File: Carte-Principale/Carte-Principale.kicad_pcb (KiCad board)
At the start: 2 copper layers, 82 parts, among them J1 Serial, J10 5V, J11 Encodeur_G, J12 Encodeur_D, J13 Moteur_Gauche, J14 Moteur_Droit, J15 PCA9685, J16 AX12, J17 I2C_Sensors, J18 LCD_TFT, J19 LCD_SD, J2 PA, J3 PG, J4 SPI2, J5 SPI3, J6 I2C2, J7 I2C3, J8 12V, J9 12VA, Q1 IRF630, Q2 BSS138, Q3 BSS138, Q4 BSS138, Q5 BSS138, SW1 RESET, SW2 Vert, SW3 Jaune, SW4 Bleu, SW5 Rouge, U1 NUCLEOH723ZG, U2 AM26LV32xD, U3 74LVC1G3157, U4 74LVC1G3157, U5 74LVC1G3157, U6 74LVC1G3157

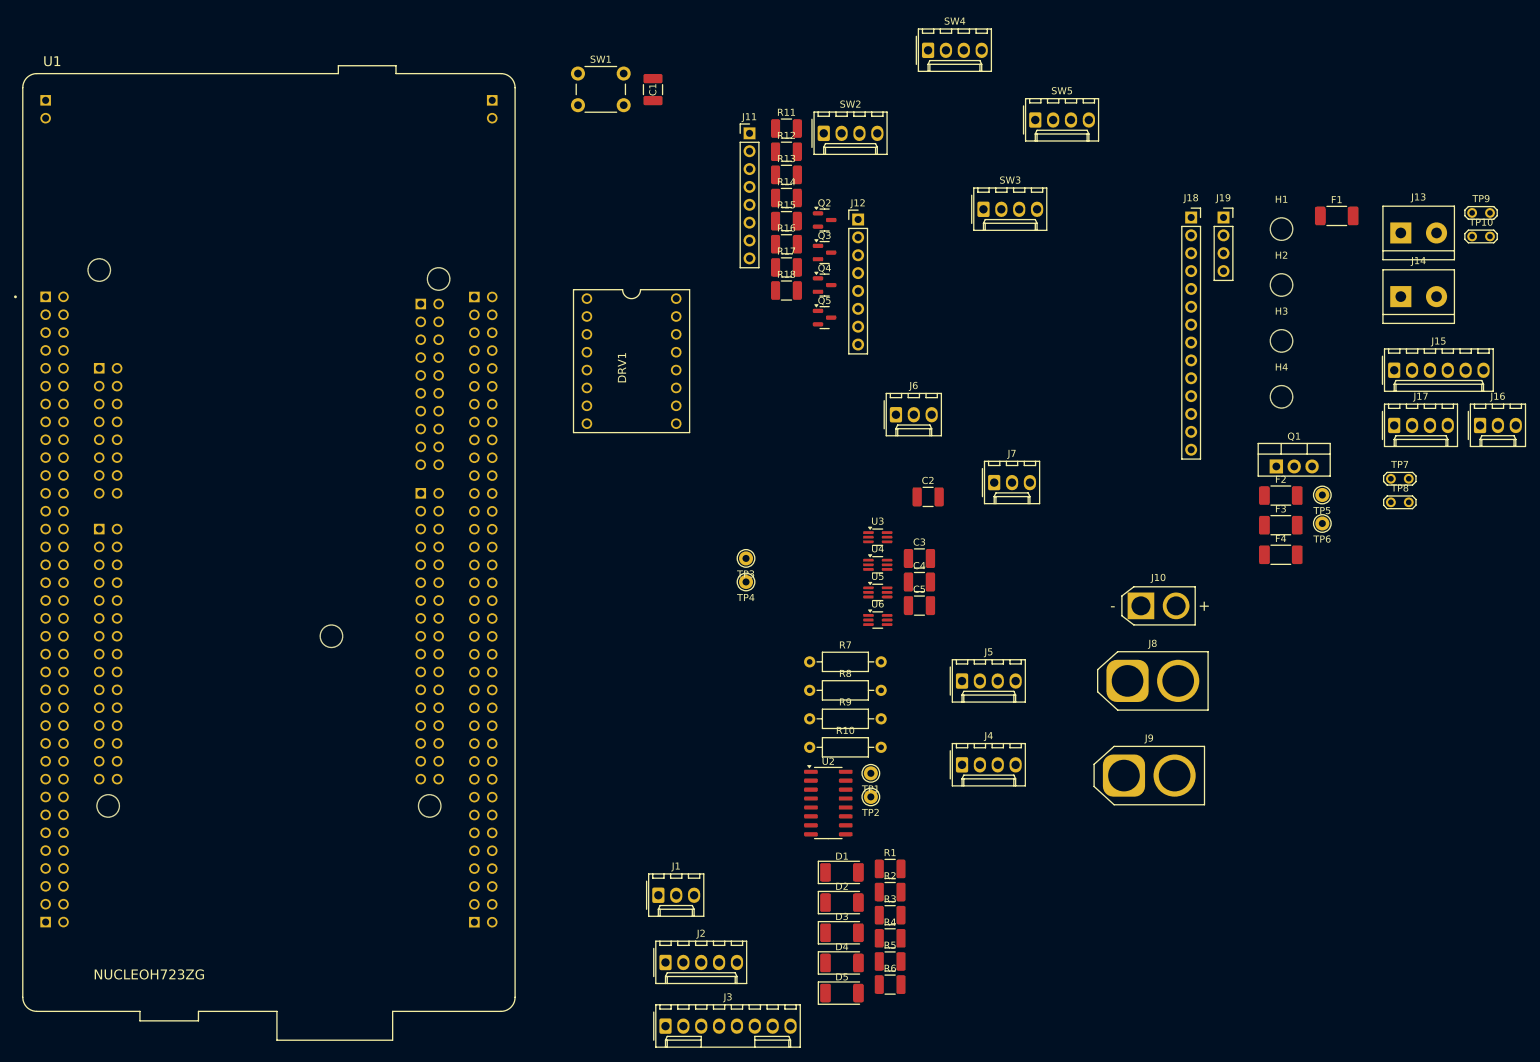
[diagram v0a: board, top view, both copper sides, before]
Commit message: Avancée PCB
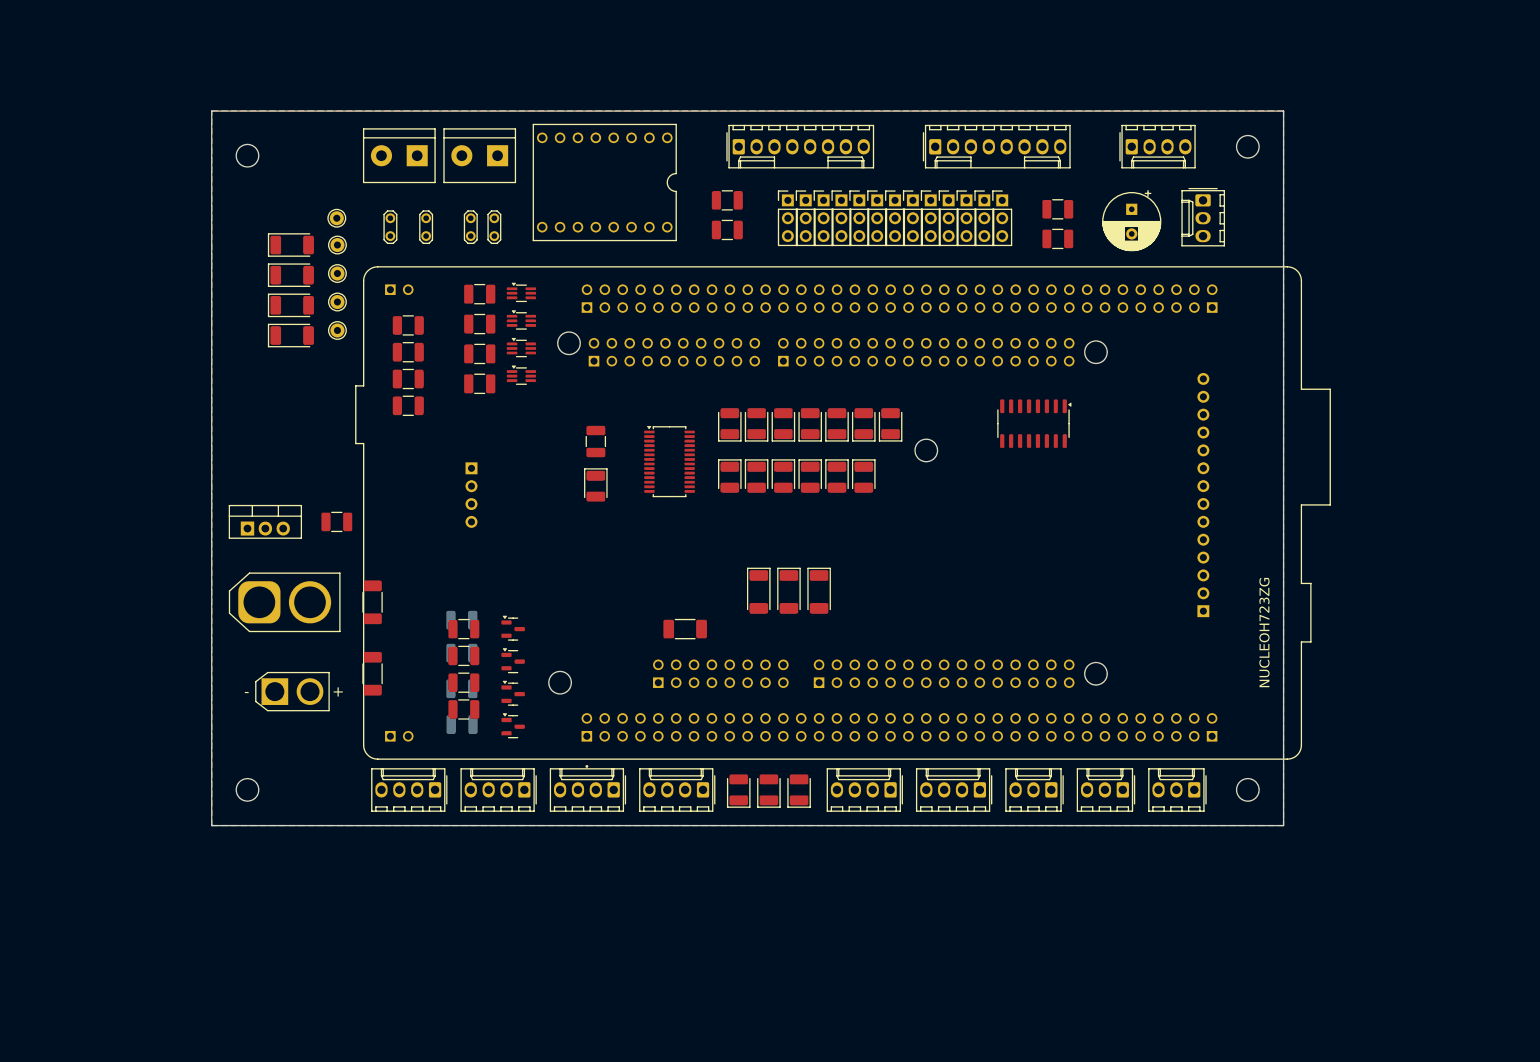
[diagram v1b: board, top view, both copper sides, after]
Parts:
- removed F4: 5A, Fuse:Fuse_2010_5025Metric_Pad1.52x2.65mm_HandSolder
- removed J16: AX12, Connector_Molex:Molex_KK-254_AE-6410-03A_1x03_P2.54mm_Vertical
- removed J17: I2C_Sensors, Connector_Molex:Molex_KK-254_AE-6410-04A_1x04_P2.54mm_Vertical
- removed J18: LCD_TFT, Connector_PinSocket_2.54mm:PinSocket_1x14_P2.54mm_Vertical
- removed J19: LCD_SD, Connector_PinSocket_2.54mm:PinSocket_1x04_P2.54mm_Vertical
- removed SW5: Rouge, Connector_Molex:Molex_KK-254_AE-6410-04A_1x04_P2.54mm_Vertical
- removed TP10: Test_DIR, TestPoint:TestPoint_2Pads_Pitch2.54mm_Drill0.8mm
- added C6: x, Capacitor_THT:CP_Radial_D8.0mm_P3.50mm, F.Cu at (189.2, 45.7)
- added D6: LED, LED_SMD:LED_2010_5025Metric_Pad1.52x2.65mm_HandSolder, F.Cu at (140.5, 100.1)
- added D7: LED, LED_SMD:LED_2010_5025Metric_Pad1.52x2.65mm_HandSolder, F.Cu at (136.2, 100.1)
- added M1: Motor_Servo, Connector_PinHeader_2.54mm:PinHeader_1x03_P2.54mm_Vertical, F.Cu at (140.3, 44.5)
- added M10: Motor_Servo, Connector_PinHeader_2.54mm:PinHeader_1x03_P2.54mm_Vertical, F.Cu at (170.8, 44.5)
- added M11: Motor_Servo, Connector_PinHeader_2.54mm:PinHeader_1x03_P2.54mm_Vertical, F.Cu at (153.0, 44.5)
- added M12: Motor_Servo, Connector_PinHeader_2.54mm:PinHeader_1x03_P2.54mm_Vertical, F.Cu at (155.6, 44.5)
- added M13: Motor_Servo, Connector_PinHeader_2.54mm:PinHeader_1x03_P2.54mm_Vertical, F.Cu at (158.1, 44.5)
- added M2: Motor_Servo, Connector_PinHeader_2.54mm:PinHeader_1x03_P2.54mm_Vertical, F.Cu at (160.7, 44.5)
- added M3: Motor_Servo, Connector_PinHeader_2.54mm:PinHeader_1x03_P2.54mm_Vertical, F.Cu at (142.9, 44.5)
- added M4: Motor_Servo, Connector_PinHeader_2.54mm:PinHeader_1x03_P2.54mm_Vertical, F.Cu at (163.2, 44.5)
- added M5: Motor_Servo, Connector_PinHeader_2.54mm:PinHeader_1x03_P2.54mm_Vertical, F.Cu at (145.4, 44.5)
- added M6: Motor_Servo, Connector_PinHeader_2.54mm:PinHeader_1x03_P2.54mm_Vertical, F.Cu at (165.7, 44.5)
- added M7: Motor_Servo, Connector_PinHeader_2.54mm:PinHeader_1x03_P2.54mm_Vertical, F.Cu at (148.0, 44.5)
- added M8: Motor_Servo, Connector_PinHeader_2.54mm:PinHeader_1x03_P2.54mm_Vertical, F.Cu at (168.3, 44.5)
- added M9: Motor_Servo, Connector_PinHeader_2.54mm:PinHeader_1x03_P2.54mm_Vertical, F.Cu at (150.5, 44.5)
- added R19: 220, LED_SMD:LED_1210_3225Metric_Pad1.42x2.65mm_HandSolder, F.Cu at (147.3, 83.8)
- added R20: 220, LED_SMD:LED_1210_3225Metric_Pad1.42x2.65mm_HandSolder, F.Cu at (143.5, 83.8)
- added R21: 220, LED_SMD:LED_1210_3225Metric_Pad1.42x2.65mm_HandSolder, F.Cu at (139.7, 83.8)
- added R22: 220, LED_SMD:LED_1210_3225Metric_Pad1.42x2.65mm_HandSolder, F.Cu at (135.9, 83.8)
- added R23: 220, LED_SMD:LED_1210_3225Metric_Pad1.42x2.65mm_HandSolder, F.Cu at (132.1, 83.8)
- added R24: x, LED_SMD:LED_1210_3225Metric_Pad1.42x2.65mm_HandSolder, F.Cu at (141.9, 128.3)
- added R25: x, LED_SMD:LED_1210_3225Metric_Pad1.42x2.65mm_HandSolder, F.Cu at (137.6, 128.3)
- added R26: x, LED_SMD:LED_1210_3225Metric_Pad1.42x2.65mm_HandSolder, F.Cu at (133.3, 128.3)
- added R27: 10k, Resistor_SMD:R_1210_3225Metric_Pad1.30x2.65mm_HandSolder, F.Cu at (94.3, 105.4)
- added R28: 10K, Resistor_SMD:R_1210_3225Metric_Pad1.30x2.65mm_HandSolder, B.Cu at (94.0, 104.1)
- added R29: 10k, Resistor_SMD:R_1210_3225Metric_Pad1.30x2.65mm_HandSolder, F.Cu at (94.3, 109.2)
- added R30: 10K, Resistor_SMD:R_1210_3225Metric_Pad1.30x2.65mm_HandSolder, B.Cu at (94.0, 108.8)
- added R31: 10k, Resistor_SMD:R_1210_3225Metric_Pad1.30x2.65mm_HandSolder, F.Cu at (94.3, 113.0)
- added R32: 10K, Resistor_SMD:R_1210_3225Metric_Pad1.30x2.65mm_HandSolder, B.Cu at (94.0, 113.9)
- added R33: 10k, Resistor_SMD:R_1210_3225Metric_Pad1.30x2.65mm_HandSolder, F.Cu at (94.3, 116.8)
- added R34: 10K, Resistor_SMD:R_1210_3225Metric_Pad1.30x2.65mm_HandSolder, B.Cu at (94.0, 119.0)
- added U7: PCA9685PW, Package_SO:TSSOP-28_4.4x9.7mm_P0.65mm, F.Cu at (123.5, 81.6)
- C1: value 0.1uF -> 100n
- C5: value 100n -> 10u
- D5: value 12V -> LED
- F2: value 2A -> 5A
- J10: value 5V -> Moteur_Gauche; footprint Connector_AMASS:AMASS_XT30U-M_1x02_P5.0mm_Vertical -> TerminalBlock:TerminalBlock_bornier-2_P5.08mm
- J11: value Encodeur_G -> Moteur_Droit; footprint Connector_PinHeader_2.54mm:PinHeader_1x08_P2.54mm_Vertical -> TerminalBlock:TerminalBlock_bornier-2_P5.08mm
- J12: value Encodeur_D -> AX12; footprint Connector_PinHeader_2.54mm:PinHeader_1x08_P2.54mm_Vertical -> Connector_Molex:Molex_KK-254_AE-6410-03A_1x03_P2.54mm_Vertical
- J13: value Moteur_Gauche -> I2C_Sensors; footprint TerminalBlock:TerminalBlock_bornier-2_P5.08mm -> Connector_Molex:Molex_KK-254_AE-6410-04A_1x04_P2.54mm_Vertical
- J14: value Moteur_Droit -> LCD_TFT; footprint TerminalBlock:TerminalBlock_bornier-2_P5.08mm -> Connector_PinSocket_2.54mm:PinSocket_1x14_P2.54mm_Vertical; moved to B.Cu
- J15: value PCA9685 -> LCD_SD; footprint Connector_Molex:Molex_KK-254_AE-6410-06A_1x06_P2.54mm_Vertical -> Connector_PinSocket_2.54mm:PinSocket_1x04_P2.54mm_Vertical; moved to B.Cu
- J2: value PA -> SPI2; footprint Connector_Molex:Molex_KK-254_AE-6410-05A_1x05_P2.54mm_Vertical -> Connector_Molex:Molex_KK-254_AE-6410-04A_1x04_P2.54mm_Vertical
- J3: value PG -> SPI3; footprint Connector_Molex:Molex_KK-254_AE-6410-08A_1x08_P2.54mm_Vertical -> Connector_Molex:Molex_KK-254_AE-6410-04A_1x04_P2.54mm_Vertical
- J4: value SPI2 -> I2C2; footprint Connector_Molex:Molex_KK-254_AE-6410-04A_1x04_P2.54mm_Vertical -> Connector_Molex:Molex_KK-254_AE-6410-03A_1x03_P2.54mm_Vertical
- J5: value SPI3 -> I2C3; footprint Connector_Molex:Molex_KK-254_AE-6410-04A_1x04_P2.54mm_Vertical -> Connector_Molex:Molex_KK-254_AE-6410-03A_1x03_P2.54mm_Vertical
- J6: value I2C2 -> 12VA; footprint Connector_Molex:Molex_KK-254_AE-6410-03A_1x03_P2.54mm_Vertical -> Connector_AMASS:AMASS_XT60-M_1x02_P7.20mm_Vertical
- J7: value I2C3 -> 5V; footprint Connector_Molex:Molex_KK-254_AE-6410-03A_1x03_P2.54mm_Vertical -> Connector_AMASS:AMASS_XT30U-M_1x02_P5.0mm_Vertical
- J8: value 12V -> Encodeur_G; footprint Connector_AMASS:AMASS_XT60-M_1x02_P7.20mm_Vertical -> Connector_Molex:Molex_KK-254_AE-6410-08A_1x08_P2.54mm_Vertical
- J9: value 12VA -> Encodeur_D; footprint Connector_AMASS:AMASS_XT60-M_1x02_P7.20mm_Vertical -> Connector_Molex:Molex_KK-254_AE-6410-08A_1x08_P2.54mm_Vertical
- R10: value 100 -> 220; footprint Resistor_THT:R_Axial_DIN0207_L6.3mm_D2.5mm_P10.16mm_Horizontal -> LED_SMD:LED_1210_3225Metric_Pad1.42x2.65mm_HandSolder
- R11, R15, R17: value 10k -> 220; footprint Resistor_SMD:R_1210_3225Metric_Pad1.30x2.65mm_HandSolder -> LED_SMD:LED_1210_3225Metric_Pad1.42x2.65mm_HandSolder
- R12, R14, R16, R18: value 10K -> 220; footprint Resistor_SMD:R_1210_3225Metric_Pad1.30x2.65mm_HandSolder -> LED_SMD:LED_1210_3225Metric_Pad1.42x2.65mm_HandSolder
- R13: footprint Resistor_SMD:R_1210_3225Metric_Pad1.30x2.65mm_HandSolder -> LED_SMD:LED_1210_3225Metric_Pad1.42x2.65mm_HandSolder
- R6: value R -> 100
- R7, R8, R9: footprint Resistor_THT:R_Axial_DIN0207_L6.3mm_D2.5mm_P10.16mm_Horizontal -> Resistor_SMD:R_1210_3225Metric_Pad1.30x2.65mm_HandSolder
- SW1: value RESET -> Vert; footprint Button_Switch_THT:SW_PUSH_6mm -> Connector_Molex:Molex_KK-254_AE-6410-04A_1x04_P2.54mm_Vertical
- SW2: value Vert -> Jaune
- SW3: value Jaune -> Bleu
- SW4: value Bleu -> Rouge
- TP6: value 12V -> Test_Gauche; footprint Connector_Pin:Pin_D1.0mm_L10.0mm -> TestPoint:TestPoint_2Pads_Pitch2.54mm_Drill0.8mm
- TP7: value Test_Gauche -> Test_Droit
- TP8: value Test_Droit -> Test_PWM
- TP9: value Test_PWM -> Test_DIR
- moved H4 157.3 mm to (63.5, 128.3)
- moved H3 149.4 mm to (63.5, 38.1)
- moved TP9 148.8 mm to (88.9, 49.5), turned to 90 degrees
- moved TP8 147.2 mm to (83.8, 49.5), turned to 90 degrees
- moved Q1 146.6 mm to (63.5, 91.1)
- moved TP5 142.0 mm to (76.3, 63.0)
- moved TP7 132.1 mm to (98.6, 49.5), turned to 90 degrees
- moved J15 131.9 mm to (95.3, 82.5), turned to 180 degrees
- moved F3 130.9 mm to (81.3, 111.8), turned to -90 degrees
- moved F2 130.0 mm to (81.3, 101.6), turned to -90 degrees
- moved TP6 127.8 mm to (95.2, 49.5), turned to 90 degrees
- moved J10 121.2 mm to (87.6, 38.1), turned to 180 degrees
- moved D1 118.6 mm to (69.8, 50.8)
- moved D2 118.6 mm to (69.8, 55.1)
- moved D3 118.6 mm to (69.8, 59.4)
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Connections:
- C1 pad 1: /NRST -> GND
- C1 pad 2: GND -> +3.3V
- C5 pad 2: +3.3V -> +5V
- D5 pad 2: Net-(D5-A) -> /Actionneurs + sensors/PWM13
- F1 pad 2: +3V3 -> +3.3V
- F2 pad 1: Net-(J8-Pin_2) -> Net-(J6-Pin_2)
- F2 pad 2: +12V -> +12VA
- F3 pad 1: Net-(J9-Pin_2) -> Net-(J7-Pin_2)
- F3 pad 2: +12VA -> +5V
- J10 pad 1: GND -> /Moteurs/MOTOR1A
- J10 pad 2: Net-(J10-Pin_2) -> /Moteurs/MOTOR1B
- J11 pad 1: +5V -> /Moteurs/MOTOR2A
- J11 pad 2: /Encodeurs/Z+_GAUCHE -> /Moteurs/MOTOR2B
- J12 pad 1: +5V -> GND
- J12 pad 2: /Encodeurs/Z+_DROITE -> +12VA
- J12 pad 3: /Encodeurs/Z-_DROITE -> /AX12_RX
- J13 pad 1: /Moteurs/MOTOR1A -> GND
- J13 pad 2: /Moteurs/MOTOR1B -> /I2C1_SCL
- J14 pad 1: /Moteurs/MOTOR2A -> +3.3V
- J14 pad 2: /Moteurs/MOTOR2B -> GND
- J15 pad 1: +5VA -> /PE3
- J15 pad 2: +5V -> /PD7
- J15 pad 3: /I2C1_SDA -> /PA6
- J15 pad 4: /I2C1_SCL -> /PA5
- J2 pad 2: /PA12 -> /PC3
- J2 pad 3: /PA11 -> /PC2
- J2 pad 4: /PA10 -> /PB10
- J3 pad 2: /PG15 -> /PB2
- J3 pad 3: /PG10 -> /PC11
- J3 pad 4: /PG9 -> /PC10
- J4 pad 2: /PC3 -> /I2C2_SDA
- J4 pad 3: /PC2 -> /I2C2_SCL
- J5 pad 2: /PB2 -> /I2C3_SDA
- J5 pad 3: /PC11 -> /I2C3_SCL
- J6 pad 2: /I2C2_SDA -> Net-(J6-Pin_2)
- J7 pad 2: /I2C3_SDA -> Net-(J7-Pin_2)
- J8 pad 1: GND -> +5V
- J8 pad 2: Net-(J8-Pin_2) -> /Encodeurs/Z+_GAUCHE
- J9 pad 1: GND -> +5V
- J9 pad 2: Net-(J9-Pin_2) -> /Encodeurs/Z+_DROITE
- R10 pad 1: /Encodeurs/A-_DROITE -> Net-(U7-LED0)
- R10 pad 2: /Encodeurs/A+_DROITE -> /Actionneurs + sensors/PWM0
- R11 pad 1: GND -> Net-(U7-LED1)
- R11 pad 2: /PE8 -> /Actionneurs + sensors/PWM1
- R12 pad 1: /PF15 -> Net-(U7-LED2)
- R12 pad 2: +5V -> /Actionneurs + sensors/PWM2
- R13 pad 1: GND -> Net-(U7-~{OE})
- R13 pad 2: /PE7 -> GND
- R14 pad 1: /PF14 -> Net-(U7-LED3)
- R14 pad 2: +5V -> /Actionneurs + sensors/PWM3
- R15 pad 1: GND -> Net-(U7-LED4)
- R15 pad 2: /PG1 -> /Actionneurs + sensors/PWM4
- R16 pad 1: /PF13 -> Net-(U7-LED5)
- R16 pad 2: +5V -> /Actionneurs + sensors/PWM5
- R17 pad 1: GND -> Net-(U7-LED6)
- R17 pad 2: /PB1 -> /Actionneurs + sensors/PWM6
- R18 pad 1: /PG0 -> Net-(U7-LED7)
- R18 pad 2: +5V -> /Actionneurs + sensors/PWM7
- R6 pad 1: +12V -> /Encodeurs/B-_GAUCHE
- R6 pad 2: Net-(D5-A) -> /Encodeurs/B+_GAUCHE
- R7 pad 1: /Encodeurs/B-_GAUCHE -> /Encodeurs/A-_GAUCHE
- R7 pad 2: /Encodeurs/B+_GAUCHE -> /Encodeurs/A+_GAUCHE
- R8 pad 1: /Encodeurs/A-_GAUCHE -> /Encodeurs/B-_DROITE
- R8 pad 2: /Encodeurs/A+_GAUCHE -> /Encodeurs/B+_DROITE
- R9 pad 1: /Encodeurs/B-_DROITE -> /Encodeurs/A-_DROITE
- R9 pad 2: /Encodeurs/B+_DROITE -> /Encodeurs/A+_DROITE
- SW1 pad 2: /NRST -> /PF15
- SW2 pad 2: /PF15 -> /PF14
- SW2 pad 3: Net-(Q2-D) -> Net-(Q3-D)
- SW3 pad 2: /PF14 -> /PF13
- SW3 pad 3: Net-(Q3-D) -> Net-(Q4-D)
- SW4 pad 2: /PF13 -> /PG0
- SW4 pad 3: Net-(Q4-D) -> Net-(Q5-D)
- TP6 pad 1: +12V -> /Encodeur_Gauche_A
- TP7 pad 1: /Encodeur_Gauche_A -> /Encodeur_Droit_A
- TP7 pad 2: /Encodeur_Gauche_B -> /Encodeur_Droit_B
- TP8 pad 1: /Encodeur_Droit_A -> /PE9
- TP8 pad 2: /Encodeur_Droit_B -> /PE11
- TP9 pad 1: /PE9 -> /PF5
- TP9 pad 2: /PE11 -> /PF4
- U1 pad CN11_1: /PC10 -> unconnected-(U1A-PC10-PadCN11_1)
- U1 pad CN11_14: /NRST -> unconnected-(U1A-NRST-PadCN11_14)
- U1 pad CN11_17: /PA15 -> unconnected-(U1A-PA15-PadCN11_17)
- U1 pad CN11_2: /PC11 -> unconnected-(U1A-PC11-PadCN11_2)
- U1 pad CN11_28: /PA0 -> unconnected-(U1A-PA0-PadCN11_28)
- U1 pad CN11_3: /PC12 -> unconnected-(U1A-PC12-PadCN11_3)
- U1 pad CN11_32: /PA4 -> unconnected-(U1A-PA4-PadCN11_32)
- U1 pad CN11_35: /PC2 -> unconnected-(U1A-PC2-PadCN11_35)
- U1 pad CN11_37: /PC3 -> unconnected-(U1A-PC3-PadCN11_37)
- U1 pad CN11_38: /PC0 -> unconnected-(U1A-PC0-PadCN11_38)
- U1 pad CN11_39: /PD4 -> unconnected-(U1A-PD4-PadCN11_39)
- U1 pad CN11_4: /PD2 -> unconnected-(U1A-PD2-PadCN11_4)
- U1 pad CN11_40: /PD3 -> unconnected-(U1A-PD3-PadCN11_40)
- U1 pad CN11_42: /PG2 -> unconnected-(U1A-PG2-PadCN11_42)
- U1 pad CN11_43: /PD6 -> unconnected-(U1A-PD6-PadCN11_43)
- U1 pad CN11_44: /PG3 -> unconnected-(U1A-PG3-PadCN11_44)
- U1 pad CN11_45: /PD7 -> unconnected-(U1A-PD7-PadCN11_45)
- U1 pad CN11_46: /PE2 -> unconnected-(U1A-PE2-PadCN11_46)
- U1 pad CN11_47: /PE3 -> unconnected-(U1A-PE3-PadCN11_47)
- U1 pad CN11_48: /PE4 -> unconnected-(U1A-PE4-PadCN11_48)
- U1 pad CN11_50: /PE5 -> unconnected-(U1A-PE5-PadCN11_50)
- U1 pad CN11_52: /PF2 -> unconnected-(U1A-PF2-PadCN11_52)
- U1 pad CN11_54: /PF8 -> unconnected-(U1A-PF8-PadCN11_54)
- U1 pad CN11_55: /PD1 -> unconnected-(U1A-PD1-PadCN11_55)
- U1 pad CN11_56: /PF9 -> unconnected-(U1A-PF9-PadCN11_56)
- U1 pad CN11_57: /PD0 -> unconnected-(U1A-PD0-PadCN11_57)
- U1 pad CN11_58: /PG1 -> unconnected-(U1A-PG1-PadCN11_58)
- U1 pad CN11_59: /PG0 -> unconnected-(U1A-PG0-PadCN11_59)
- U1 pad CN11_62: /PE6 -> unconnected-(U1A-PE6-PadCN11_62)
- U1 pad CN11_63: /PG9 -> unconnected-(U1A-PG9-PadCN11_63)
- U1 pad CN11_64: /PG15 -> unconnected-(U1A-PG15-PadCN11_64)
- U1 pad CN11_65: /PG12 -> unconnected-(U1A-PG12-PadCN11_65)
- U1 pad CN11_66: /PG10 -> unconnected-(U1A-PG10-PadCN11_66)
- U1 pad CN12_11: /PA5 -> unconnected-(U1B-PA5-PadCN12_11)
- U1 pad CN12_12: /PA12 -> unconnected-(U1B-PA12-PadCN12_12)
- U1 pad CN12_13: /PA6 -> unconnected-(U1B-PA6-PadCN12_13)
- U1 pad CN12_14: /PA11 -> unconnected-(U1B-PA11-PadCN12_14)
- U1 pad CN12_16: /PB12 -> unconnected-(U1B-PB12-PadCN12_16)
- U1 pad CN12_18: /PB11 -> unconnected-(U1B-PB11-PadCN12_18)
- U1 pad CN12_19: /PC7 -> unconnected-(U1B-PC7-PadCN12_19)
- U1 pad CN12_2: /PC8 -> unconnected-(U1B-PC8-PadCN12_2)
- U1 pad CN12_21: /PA9 -> unconnected-(U1B-PA9-PadCN12_21)
- U1 pad CN12_22: /PB2 -> unconnected-(U1B-PB2-PadCN12_22)
- U1 pad CN12_24: /PB1 -> unconnected-(U1B-PB1-PadCN12_24)
- U1 pad CN12_25: /PB10 -> unconnected-(U1B-PB10-PadCN12_25)
- U1 pad CN12_26: /PB15 -> unconnected-(U1B-PB15-PadCN12_26)
- U1 pad CN12_28: /PB14 -> unconnected-(U1B-PB14-PadCN12_28)
- U1 pad CN12_29: /PB5 -> unconnected-(U1B-PB5-PadCN12_29)
- U1 pad CN12_3: /PB8 -> unconnected-(U1B-PB8-PadCN12_3)
- U1 pad CN12_30: /PB13 -> unconnected-(U1B-PB13-PadCN12_30)
- U1 pad CN12_33: /PA10 -> unconnected-(U1B-PA10-PadCN12_33)
- U1 pad CN12_36: /PF5 -> unconnected-(U1B-PF5-PadCN12_36)
- U1 pad CN12_38: /PF4 -> unconnected-(U1B-PF4-PadCN12_38)
- U1 pad CN12_4: /PC6 -> unconnected-(U1B-PC6-PadCN12_4)
- U1 pad CN12_40: /PE8 -> unconnected-(U1B-PE8-PadCN12_40)
- U1 pad CN12_41: /PD13 -> unconnected-(U1B-PD13-PadCN12_41)
- U1 pad CN12_42: /PF10 -> unconnected-(U1B-PF10-PadCN12_42)
- U1 pad CN12_43: /PD12 -> unconnected-(U1B-PD12-PadCN12_43)
- U1 pad CN12_44: /PE7 -> unconnected-(U1B-PE7-PadCN12_44)
- U1 pad CN12_45: /PD11 -> unconnected-(U1B-PD11-PadCN12_45)
- U1 pad CN12_46: /PD14 -> unconnected-(U1B-PD14-PadCN12_46)
- U1 pad CN12_47: /PE10 -> unconnected-(U1B-PE10-PadCN12_47)
- U1 pad CN12_48: /PD15 -> unconnected-(U1B-PD15-PadCN12_48)
- U1 pad CN12_49: /PE12 -> unconnected-(U1B-PE12-PadCN12_49)
- U1 pad CN12_5: /PB9 -> unconnected-(U1B-PB9-PadCN12_5)
- U1 pad CN12_50: /PF14 -> unconnected-(U1B-PF14-PadCN12_50)
- U1 pad CN12_51: /PE14 -> unconnected-(U1B-PE14-PadCN12_51)
- U1 pad CN12_52: /PE9 -> unconnected-(U1B-PE9-PadCN12_52)
- U1 pad CN12_53: /PE15 -> unconnected-(U1B-PE15-PadCN12_53)
- U1 pad CN12_55: /PE13 -> unconnected-(U1B-PE13-PadCN12_55)
- U1 pad CN12_56: /PE11 -> unconnected-(U1B-PE11-PadCN12_56)
- U1 pad CN12_57: /PF13 -> unconnected-(U1B-PF13-PadCN12_57)
- U1 pad CN12_58: /PF3 -> unconnected-(U1B-PF3-PadCN12_58)
- U1 pad CN12_60: /PF15 -> unconnected-(U1B-PF15-PadCN12_60)
- U1 pad CN12_61: /PG14 -> unconnected-(U1B-PG14-PadCN12_61)
- U1 pad CN12_64: /PE0 -> unconnected-(U1B-PE0-PadCN12_64)
- U1 pad CN12_66: /PG8 -> unconnected-(U1B-PG8-PadCN12_66)
- U1 pad CN12_68: /PG5 -> unconnected-(U1B-PG5-PadCN12_68)
- U1 pad CN12_69: /PG4 -> unconnected-(U1B-PG4-PadCN12_69)
- U1 pad CN12_70: /PG6 -> unconnected-(U1B-PG6-PadCN12_70)
- U1 pad CN8_5: /NRST -> unconnected-(U1C-NRST_CN8-PadCN8_5)
- U1 pad CN8_7: +3V3 -> Net-(U1A-3V3)
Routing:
- added copper zone on B.Cu, net GND
- added copper zone on F.Cu, net GND
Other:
- board outline added: 152.4 x 101.6 mm

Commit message: avancée
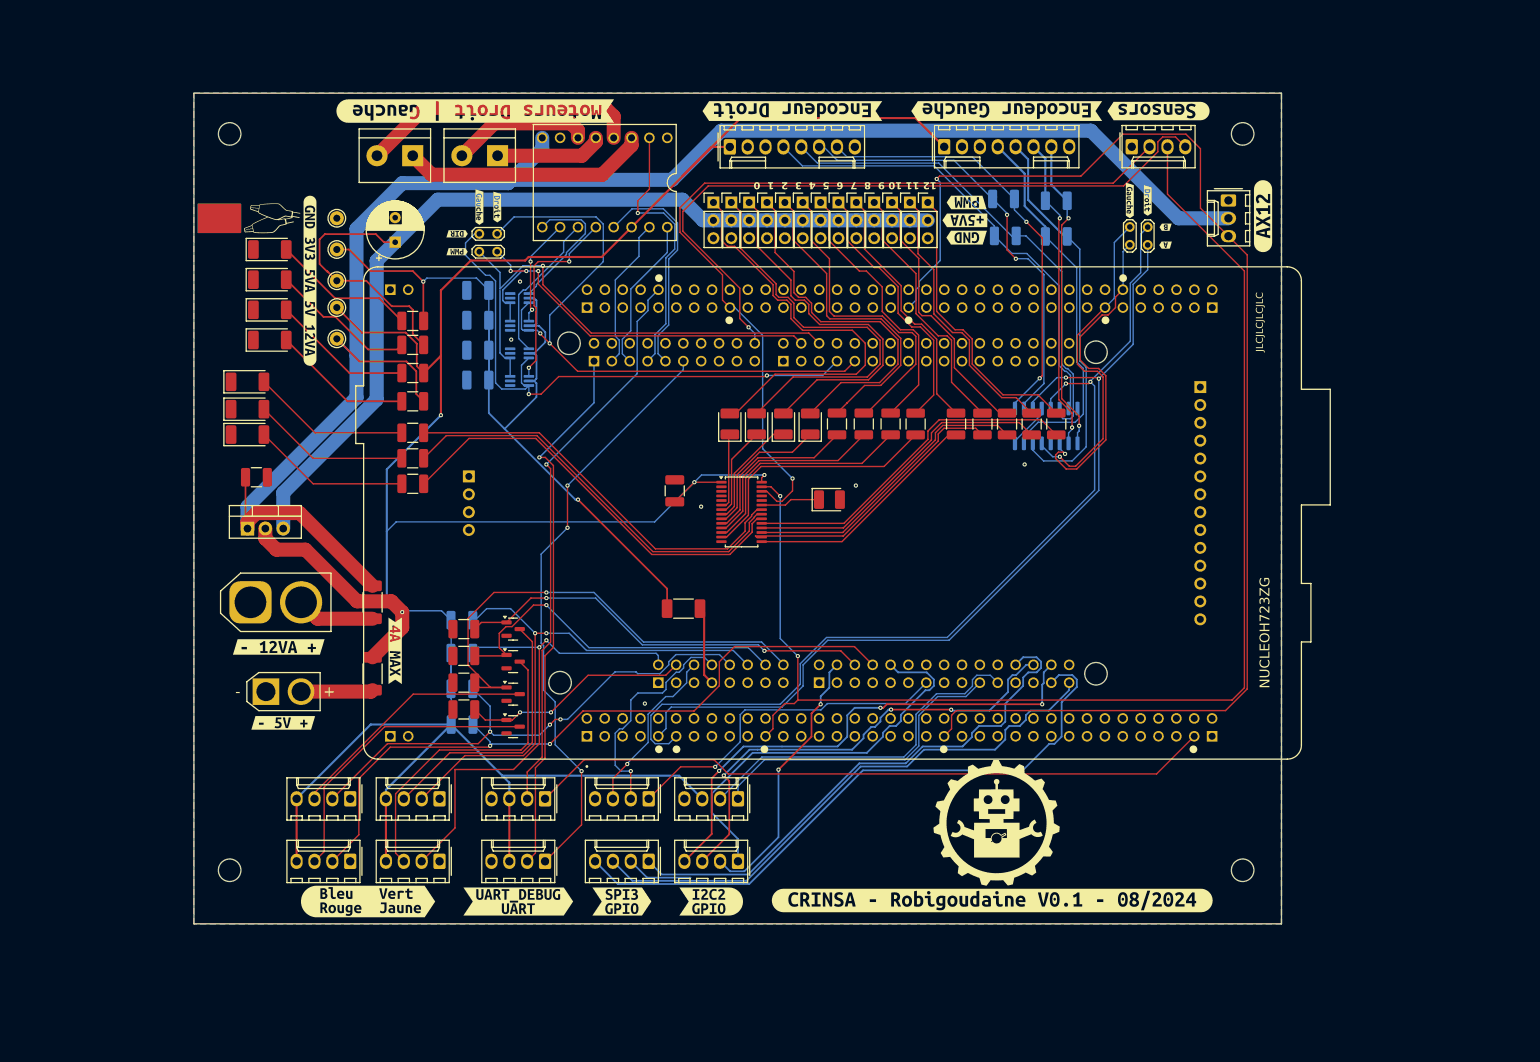
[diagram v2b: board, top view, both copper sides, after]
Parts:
- removed the J3 at (154.9, 128.3)
- removed the J4 at (188.0, 128.3)
- added G***: LOGO, LOGO, F.Cu at (67.0, 47.0)
- added G0: LOGO, LOGO, F.Cu at (170.0, 133.0)
- added J10: SPI3, Connector_Molex:Molex_KK-254_AE-6410-04A_1x04_P2.54mm_Vertical, F.Cu at (120.5, 129.5)
- added J8: I2C2, Connector_Molex:Molex_KK-254_AE-6410-04A_1x04_P2.54mm_Vertical, F.Cu at (133.2, 129.5)
- added J9: GPIO, Connector_Molex:Molex_KK-254_AE-6410-04A_1x04_P2.54mm_Vertical, F.Cu at (120.5, 138.4)
- added kibuzzard-1: G***, kibuzzard-66C08CAE, F.Cu at (72.4, 55.9)
- added kibuzzard-10: G***, kibuzzard-66C08EB4, F.Cu at (102.0, 144.1)
- added kibuzzard-11: G***, kibuzzard-66C46925, F.Cu at (129.4, 144.1)
- added kibuzzard-13: G***, kibuzzard-66C08BB8, F.Cu at (141.0, 31.8)
- added kibuzzard-14: G***, kibuzzard-66C08BD9, F.Cu at (171.4, 31.8)
- added kibuzzard-15: G***, kibuzzard-66C34407, F.Cu at (165.8, 49.8)
- added kibuzzard-16: G***, kibuzzard-66C3440D, F.Cu at (165.8, 44.8)
- added kibuzzard-17: G***, kibuzzard-66C0927B, F.Cu at (189.0, 44.5)
- added kibuzzard-18: G***, kibuzzard-66C34414, F.Cu at (165.5, 47.3)
- added kibuzzard-19: G***, kibuzzard-66C3235E, F.Cu at (169.4, 144.0)
- added kibuzzard-2: G***, kibuzzard-66C08D4F, F.Cu at (67.9, 108.0)
- added kibuzzard-20: G***, kibuzzard-66C32535, F.Cu at (193.0, 31.8)
- added kibuzzard-21: G***, kibuzzard-66C09269, F.Cu at (191.5, 44.5)
- added kibuzzard-22: G***, kibuzzard-66C0929D, F.Cu at (194.0, 50.8)
- added kibuzzard-23: G***, kibuzzard-66C3253B, F.Cu at (207.9, 46.7)
- added kibuzzard-24: G***, kibuzzard-66C09293, F.Cu at (194.0, 48.3)
- added kibuzzard-25: G***, kibuzzard-66C091C7, B.Cu at (193.0, 33.0)
- added kibuzzard-26: G***, kibuzzard-66C0922C, B.Cu at (207.2, 47.0)
- added kibuzzard-27: G***, kibuzzard-66C091DE, B.Cu at (171.4, 33.0)
- added kibuzzard-28: G***, kibuzzard-66C091DE, B.Cu at (141.0, 33.0)
- added kibuzzard-29: G***, kibuzzard-66C09378, B.Cu at (129.4, 134.0)
- added kibuzzard-3: G***, kibuzzard-66C08D66, F.Cu at (68.6, 118.7)
- added kibuzzard-30: G***, kibuzzard-66C09044, B.Cu at (116.7, 134.0)
- added kibuzzard-31: G***, kibuzzard-66C09044, B.Cu at (116.7, 142.9)
- added kibuzzard-32: G***, kibuzzard-66C090AC, B.Cu at (96.5, 33.0)
- added kibuzzard-33: G***, kibuzzard-66C09018, B.Cu at (102.0, 134.0)
- added kibuzzard-34: G***, kibuzzard-66C09018, B.Cu at (102.0, 142.9)
- added kibuzzard-35: G***, kibuzzard-66C090AC, B.Cu at (84.5, 33.0)
- added kibuzzard-36: G***, kibuzzard-66C08FE4, B.Cu at (87.0, 134.0)
- added kibuzzard-37: G***, kibuzzard-66C08FE4, B.Cu at (74.3, 134.0)
- added kibuzzard-38: G***, kibuzzard-66C08FE4, B.Cu at (87.0, 142.9)
- added kibuzzard-39: G***, kibuzzard-66C08FE4, B.Cu at (74.3, 142.9)
- added kibuzzard-4: G***, kibuzzard-66C08EFC, F.Cu at (80.6, 144.1)
- added kibuzzard-5: G***, kibuzzard-66C08F7C, F.Cu at (95.9, 31.8)
- added kibuzzard-6: G***, kibuzzard-66C09269, F.Cu at (99.0, 45.4)
- added kibuzzard-66C478F6: G***, kibuzzard-66C478F6, F.Cu at (84.5, 108.5)
- added kibuzzard-66C48662: G***, kibuzzard-66C48662, F.Cu at (116.7, 144.1)
- added kibuzzard-7: G***, kibuzzard-66C0927B, F.Cu at (96.5, 45.4)
- added kibuzzard-8: G***, kibuzzard-66C092E0, F.Cu at (93.3, 49.2)
- added kibuzzard-9: G***, kibuzzard-66C092F4, F.Cu at (93.3, 51.8)
- C3, C4, U5: moved to B.Cu
- C5: renamed from C1; moved to B.Cu
- C6: renamed from C2; moved to B.Cu
- J11: renamed from J2; value SPI2 -> GPIO
- J5: value I2C3 -> UART_Debug; footprint Connector_Molex:Molex_KK-254_AE-6410-03A_1x03_P2.54mm_Vertical -> Connector_Molex:Molex_KK-254_AE-6410-04A_1x04_P2.54mm_Vertical
- J6: renamed from J1; value Serial -> UART; footprint Connector_Molex:Molex_KK-254_AE-6410-03A_1x03_P2.54mm_Vertical -> Connector_Molex:Molex_KK-254_AE-6410-04A_1x04_P2.54mm_Vertical
- R16: renamed from R19; footprint LED_SMD:LED_1210_3225Metric_Pad1.42x2.65mm_HandSolder -> Resistor_SMD:R_1210_3225Metric_Pad1.30x2.65mm_HandSolder
- R18: renamed from R17; footprint LED_SMD:LED_1210_3225Metric_Pad1.42x2.65mm_HandSolder -> Resistor_SMD:R_1210_3225Metric_Pad1.30x2.65mm_HandSolder
- R19: renamed from R16; footprint LED_SMD:LED_1210_3225Metric_Pad1.42x2.65mm_HandSolder -> Resistor_SMD:R_1210_3225Metric_Pad1.30x2.65mm_HandSolder
- R2: renamed from R24; footprint LED_SMD:LED_1210_3225Metric_Pad1.42x2.65mm_HandSolder -> Resistor_SMD:R_1210_3225Metric_Pad1.30x2.65mm_HandSolder
- R20: renamed from R18; footprint LED_SMD:LED_1210_3225Metric_Pad1.42x2.65mm_HandSolder -> Resistor_SMD:R_1210_3225Metric_Pad1.30x2.65mm_HandSolder
- R22: renamed from R15; footprint LED_SMD:LED_1210_3225Metric_Pad1.42x2.65mm_HandSolder -> Resistor_SMD:R_1210_3225Metric_Pad1.30x2.65mm_HandSolder
- R23: footprint LED_SMD:LED_1210_3225Metric_Pad1.42x2.65mm_HandSolder -> Resistor_SMD:R_1210_3225Metric_Pad1.30x2.65mm_HandSolder
- R24: renamed from R22; footprint LED_SMD:LED_1210_3225Metric_Pad1.42x2.65mm_HandSolder -> Resistor_SMD:R_1210_3225Metric_Pad1.30x2.65mm_HandSolder
- R25: renamed from R20; footprint LED_SMD:LED_1210_3225Metric_Pad1.42x2.65mm_HandSolder -> Resistor_SMD:R_1210_3225Metric_Pad1.30x2.65mm_HandSolder
- R26: renamed from R21; footprint LED_SMD:LED_1210_3225Metric_Pad1.42x2.65mm_HandSolder -> Resistor_SMD:R_1210_3225Metric_Pad1.30x2.65mm_HandSolder
- R27: renamed from R9; moved to B.Cu
- R28: renamed from R6; moved to B.Cu
- R29: renamed from R8; moved to B.Cu
- R30: renamed from R7; moved to B.Cu
- R5: renamed from R25; footprint LED_SMD:LED_1210_3225Metric_Pad1.42x2.65mm_HandSolder -> Resistor_SMD:R_1210_3225Metric_Pad1.30x2.65mm_HandSolder
- R6: renamed from R26; footprint LED_SMD:LED_1210_3225Metric_Pad1.42x2.65mm_HandSolder -> Resistor_SMD:R_1210_3225Metric_Pad1.30x2.65mm_HandSolder
- TP6: value Test_Gauche -> Test_PWM
- TP7: value Test_Droit -> Test_DIR
- TP8: value Test_PWM -> Test_Gauche
- TP9: value Test_DIR -> Test_Droit
- U3: renamed from U2; moved to B.Cu
- U4: renamed from U6; moved to B.Cu
- U6: renamed from U4; moved to B.Cu
- U7: renamed from U3; moved to B.Cu
- moved TP8 105.1 mm to (189.0, 50.8)
- moved C1 104.8 mm to (84.5, 50.4), turned to 90 degrees
- moved TP9 102.6 mm to (191.5, 50.8)
- moved J6 92.9 mm to (105.8, 138.4)
- moved D2 84.3 mm to (63.5, 77.8), turned to 0 degrees
- moved D3 81.3 mm to (63.5, 74.1), turned to 0 degrees
- moved D1 78.6 mm to (63.5, 70.2), turned to 0 degrees
- moved J5 72.0 mm to (105.8, 129.5)
- moved R2 70.1 mm to (87.0, 84.8), turned to 180 degrees
- moved R5 69.2 mm to (87.0, 81.1), turned to 180 degrees
- moved R6 68.7 mm to (87.0, 77.5), turned to 180 degrees
- moved SW2 51.2 mm to (78.1, 138.4)
- moved R23 47.0 mm to (178.5, 76.2), turned to 90 degrees
- moved R29 39.8 mm to (171.2, 49.5)
- moved R24 39.8 mm to (175.0, 76.2), turned to 90 degrees
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- renumbered C6 to C1, C5 to C2, D7 to D1, D5 to D2, D6 to D3, D3 to D4, D2 to D5, D1 to D6, D4 to D7, F3 to F1, F1 to F3, H3 to H1, H4 to H2, H1 to H3, H2 to H4, J10 to J1, J8 to J12, J13 to J17, J6 to J2, J12 to J20, J14 to J21, J15 to J22, J7 to J3, J11 to J4, J9 to J7, M2 to M10, M8 to M11, M11 to M13, M7 to M2, M5 to M4, M9 to M5, M4 to M6, M13 to M7, M10 to M8, M6 to M9, Q3 to Q2, Q2 to Q3, R2 to R1, R31 to R10, R29 to R11, R33 to R12, R12 to R13, R10 to R14, R11 to R15, R14 to R17, R13 to R21, R5 to R3, R32 to R31, R30 to R32, R28 to R33, R3 to R4, R1 to R7, R4 to R8, R27 to R9, SW3 to SW1, SW4 to SW2, SW2 to SW3, SW1 to SW4, TP2 to TP1, TP4 to TP2, TP1 to TP3, TP3 to TP4, U7 to U1, U1 to U2
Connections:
- DRV1 pad EN1: /PF8 -> /PB13
- DRV1 pad EN2: /PF9 -> /PB15
- DRV1 pad FLT: /PE6 -> /PB12
- DRV1 pad RST: /PF10 -> /PA15
- F3 pad 1: Net-(U1A-3V3) -> Net-(U2C-3V3_CN8)
- J11 pad 1: GND -> /PD3
- J11 pad 2: /PC3 -> /PD6
- J11 pad 3: /PC2 -> /PF7
- J11 pad 4: /PB10 -> /PF9
- J5 pad 1: GND -> /DEBUG_RX
- J5 pad 2: /I2C3_SDA -> /DEBUG_TX
- J5 pad 3: /I2C3_SCL -> +5V
- J6 pad 1: GND -> /PC7
- J6 pad 2: /DEBUG_TX -> /PC6
- J6 pad 3: /DEBUG_RX -> +5V
- Q2 pad 1: /PE7 -> /PG2
- Q3 pad 1: /PE8 -> /PD5
- Q4 pad 1: /PG1 -> /PG3
- Q5 pad 1: /PB1 -> /PC9
- R10 pad 2: /PG1 -> /PG3
- R11 pad 2: /PE7 -> /PG2
- R12 pad 2: /PB1 -> /PC9
- R31 pad 1: /PF13 -> /PC12
- R32 pad 1: /PF14 -> /PC8
- R33 pad 1: /PF15 -> /PD2
- R34 pad 1: /PG0 -> /PD4
- R9 pad 2: /PE8 -> /PD5
- SW1 pad 2: /PF13 -> /PC12
- SW2 pad 2: /PG0 -> /PD4
- SW3 pad 2: /PF14 -> /PC8
- SW4 pad 2: /PF15 -> /PD2
- TP6 pad 1: /Encodeur_Gauche_A -> /PE9
- TP6 pad 2: /Encodeur_Gauche_B -> /PE11
- TP7 pad 1: /Encodeur_Droit_A -> /PF5
- TP7 pad 2: /Encodeur_Droit_B -> /PF4
- TP8 pad 1: /PE9 -> /Encodeur_Gauche_A
- TP8 pad 2: /PE11 -> /Encodeur_Gauche_B
- TP9 pad 1: /PF5 -> /Encodeur_Droit_A
- TP9 pad 2: /PF4 -> /Encodeur_Droit_B
- U2 pad CN10_10: /PE13 -> unconnected-(U2F-D3/TIMER_A_PWM3-PadCN10_10)
- U2 pad CN10_11: /Encodeur_Droit_A -> /PF6
- U2 pad CN10_12: /PG14 -> unconnected-(U2F-D2/IO-PadCN10_12)
- U2 pad CN10_14: /I2C1_SCL -> unconnected-(U2F-D1/USART_A_TX-PadCN10_14)
- U2 pad CN10_15: /PB2 -> unconnected-(U2F-D27/QSPI_CLK-PadCN10_15)
- U2 pad CN10_16: /I2C1_SDA -> unconnected-(U2F-D0/USART_A_RX-PadCN10_16)
- U2 pad CN10_2: /PG12 -> unconnected-(U2F-D7/IO-PadCN10_2)
- U2 pad CN10_25: /PE2 -> unconnected-(U2F-D31/QSPI_BK1_IO2-PadCN10_25)
- U2 pad CN10_8: /PE14 -> unconnected-(U2F-D4/IO-PadCN10_8)
- U2 pad CN11_16: Net-(U1A-3V3) -> unconnected-(U2A-3V3-PadCN11_16)
- U2 pad CN11_51: /I2C2_SCL -> unconnected-(U2A-PF1-PadCN11_51)
- U2 pad CN11_53: /I2C2_SDA -> unconnected-(U2A-PF0-PadCN11_53)
- U2 pad CN12_1: /I2C3_SDA -> unconnected-(U2B-PC9-PadCN12_1)
- U2 pad CN12_23: /I2C3_SCL -> unconnected-(U2B-PA8-PadCN12_23)
- U2 pad CN7_13: /PB5 -> unconnected-(U2E-D22/I2S_B_SD/SPI_B_MOSI-PadCN7_13)
- U2 pad CN7_14: /PB5 -> unconnected-(U2E-D11/SPI_A_MOSI/TIM_E_PWM1-PadCN7_14)
- U2 pad CN7_16: /PD14 -> unconnected-(U2E-D10/SPI_A_CS/TIM_B_PWM3-PadCN7_16)
- U2 pad CN7_18: /PD15 -> unconnected-(U2E-D9/TIMER_B_PWM2-PadCN7_18)
- U2 pad CN7_2: /PB8 -> unconnected-(U2E-D15/I2C_A_SCL-PadCN7_2)
- U2 pad CN7_4: /PB9 -> unconnected-(U2E-D14/I2C_A_SDA-PadCN7_4)
- U2 pad CN8_4: /I2C3_SDA -> /PC9
- U2 pad CN8_7: Net-(U1A-3V3) -> Net-(U2C-3V3_CN8)
- U2 pad CN9_1: /AX12_RX -> unconnected-(U2D-A0/ADC12_INP15-PadCN9_1)
- U2 pad CN9_11: /PF10 -> unconnected-(U2D-A5/ADC3_INP6/I2C1_SCL-PadCN9_11)
- U2 pad CN9_15: /PE9 -> unconnected-(U2D-D71/COMP2_INP-PadCN9_15)
- U2 pad CN9_20: /PE6 -> unconnected-(U2D-D59/SAI_A_SD-PadCN9_20)
- U2 pad CN9_26: /Encodeur_Droit_B -> /PF7
- U2 pad CN9_3: /PC0 -> unconnected-(U2D-A1/ADC123_INP10-PadCN9_3)
- U2 pad CN9_5: /PC3 -> unconnected-(U2D-A2/ADC12_INP13-PadCN9_5)
- U2 pad CN9_6: /AX12_RX -> /PD5
- U2 pad CN9_7: /PB1 -> unconnected-(U2D-A3/ADC12_INP5-PadCN9_7)
- U2 pad CN9_9: /PC2 -> unconnected-(U2D-A4/ADC123_INP12/I2C1_SDA-PadCN9_9)
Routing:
- net +5V: track 0.00 -> 400.4 mm, vias 0 -> 4
- net +12VA: track 0.00 -> 245.0 mm
- net /AX12_RX: track 0.00 -> 187.9 mm, vias 0 -> 1
- net /I2C1_SDA: track 0.00 -> 186.8 mm, vias 0 -> 2
- net +5VA: track 0.00 -> 163.4 mm
- net /Encodeur_Droit_B: track 0.00 -> 135.2 mm, vias 0 -> 2
- net /Encodeur_Droit_A: track 0.00 -> 130.0 mm, vias 0 -> 2
- net +3.3V: track 0.00 -> 127.6 mm, vias 0 -> 2
- net /I2C1_SCL: track 0.00 -> 123.2 mm, vias 0 -> 1
- net /PD4: track 0.00 -> 101.3 mm, vias 0 -> 2
- net /PF3: track 0.00 -> 100.2 mm, vias 0 -> 1
- net /DEBUG_RX: track 0.00 -> 97.6 mm
- net /PF5: track 0.00 -> 91.3 mm, vias 0 -> 2
- net /PD1: track 0.00 -> 89.7 mm
- net /PC7: track 0.00 -> 84.0 mm, vias 0 -> 3
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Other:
- board size 152.4 x 101.6 mm -> 154.6 x 118.1 mm
- board text added: "12 11 10 9 8 7 6 5 4 3 2 1 0"
- board text added: "JLCJLCJLCJLC"
